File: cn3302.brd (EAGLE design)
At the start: 54 x 20 mm, 20 parts, among them M1 CN3302SOP-8, T1 AOD9N50

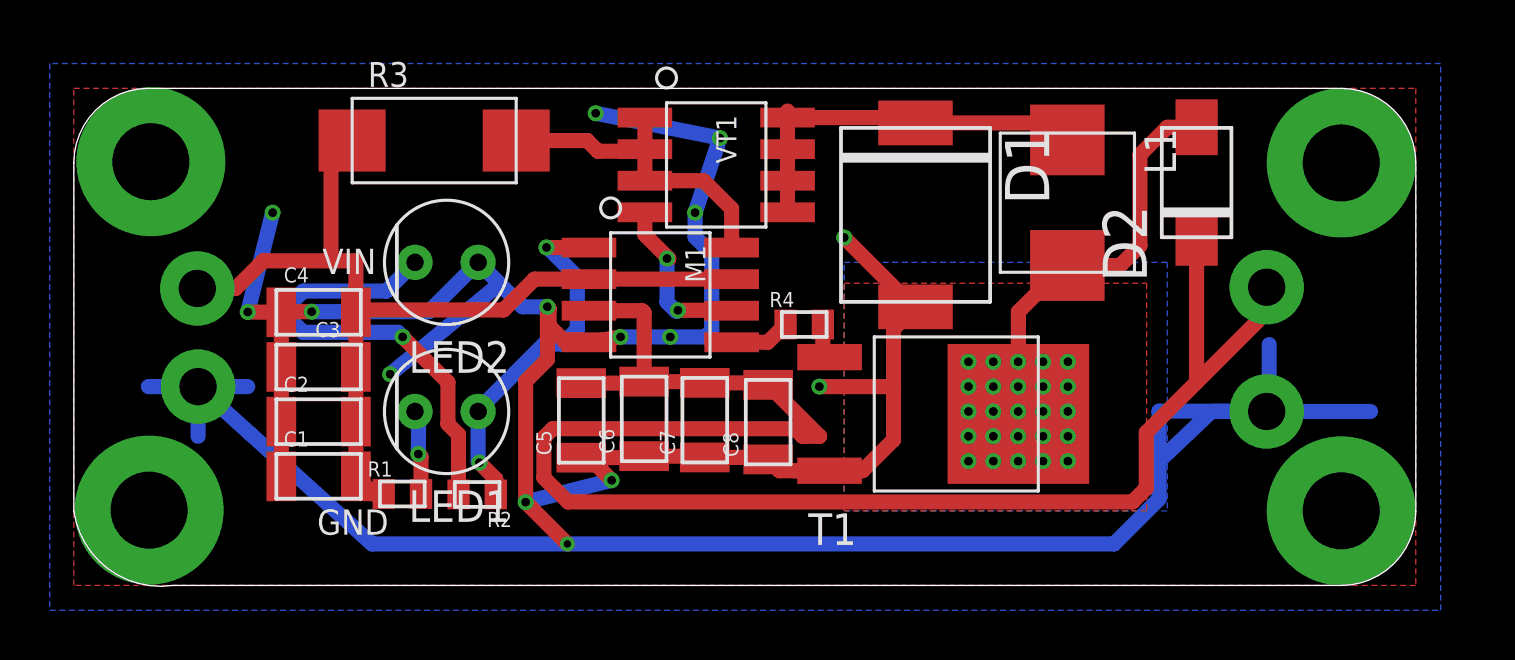
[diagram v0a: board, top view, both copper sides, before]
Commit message: Исправил плату
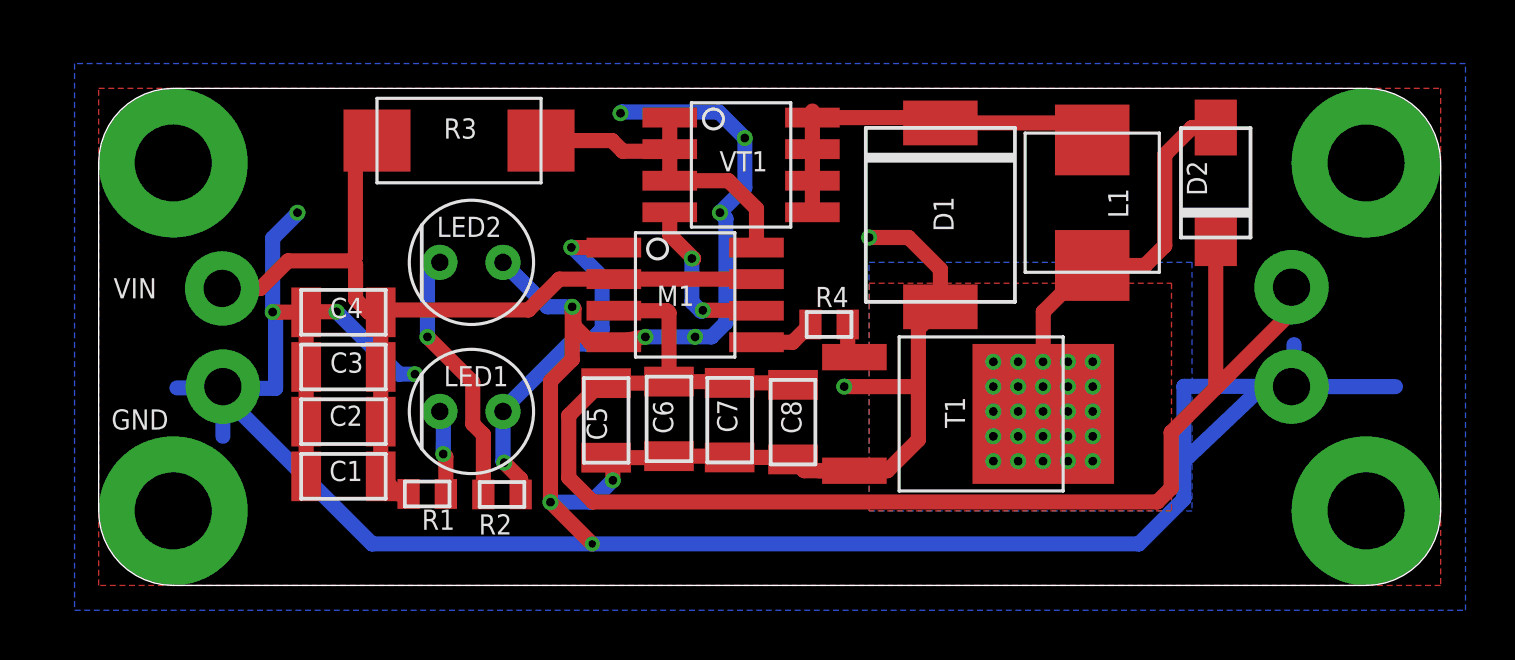
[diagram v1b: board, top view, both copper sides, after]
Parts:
- moved C1 1.00 mm to (10.8, 5.39)
- moved C2 1.00 mm to (10.8, 7.59)
- moved C3 1.00 mm to (10.8, 9.79)
- moved C4 1.00 mm to (10.8, 12.0)
- moved C5 1.00 mm to (21.4, 7.64)
- moved C6 1.00 mm to (23.9, 7.70)
- moved C7 1.00 mm to (26.4, 7.65)
- moved C8 1.00 mm to (28.9, 7.57)
- moved D1 1.00 mm to (34.9, 15.9)
- moved L1 1.00 mm to (41.0, 16.4)
- moved LED1 1.00 mm to (16.0, 8.00)
- moved LED2 1.00 mm to (16.0, 14.0)
- moved M1 1.00 mm to (24.6, 12.7)
- moved R1 1.00 mm to (14.2, 4.68)
- moved R2 1.00 mm to (17.2, 4.66)
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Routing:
- net 8.4V: track 69.5 -> 59.3 mm
- net N$2: track 18.4 -> 10.5 mm
- net GND: track 163.4 -> 158.0 mm
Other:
- outline, holes or cut-outs redrawn
